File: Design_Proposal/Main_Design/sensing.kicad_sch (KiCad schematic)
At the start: 13 parts, among them IC2 TMP102AIDRLR, J10 Conn_01x03_Male, J11 Conn_01x05_Male

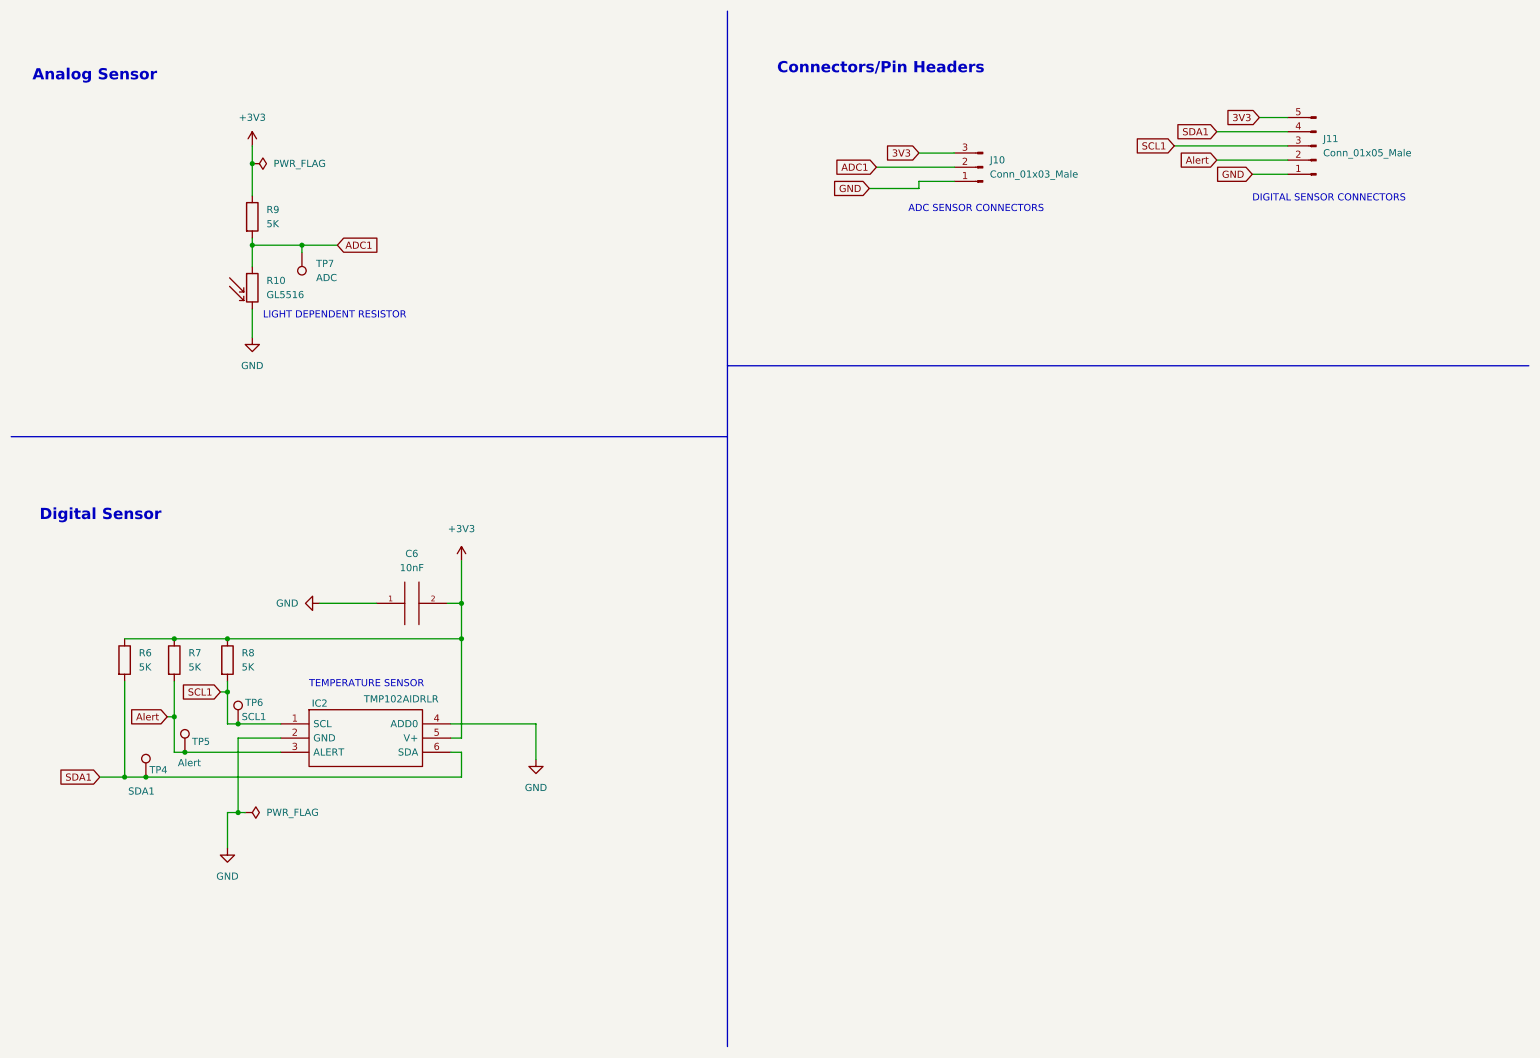
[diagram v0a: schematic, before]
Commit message: Final PCB Design
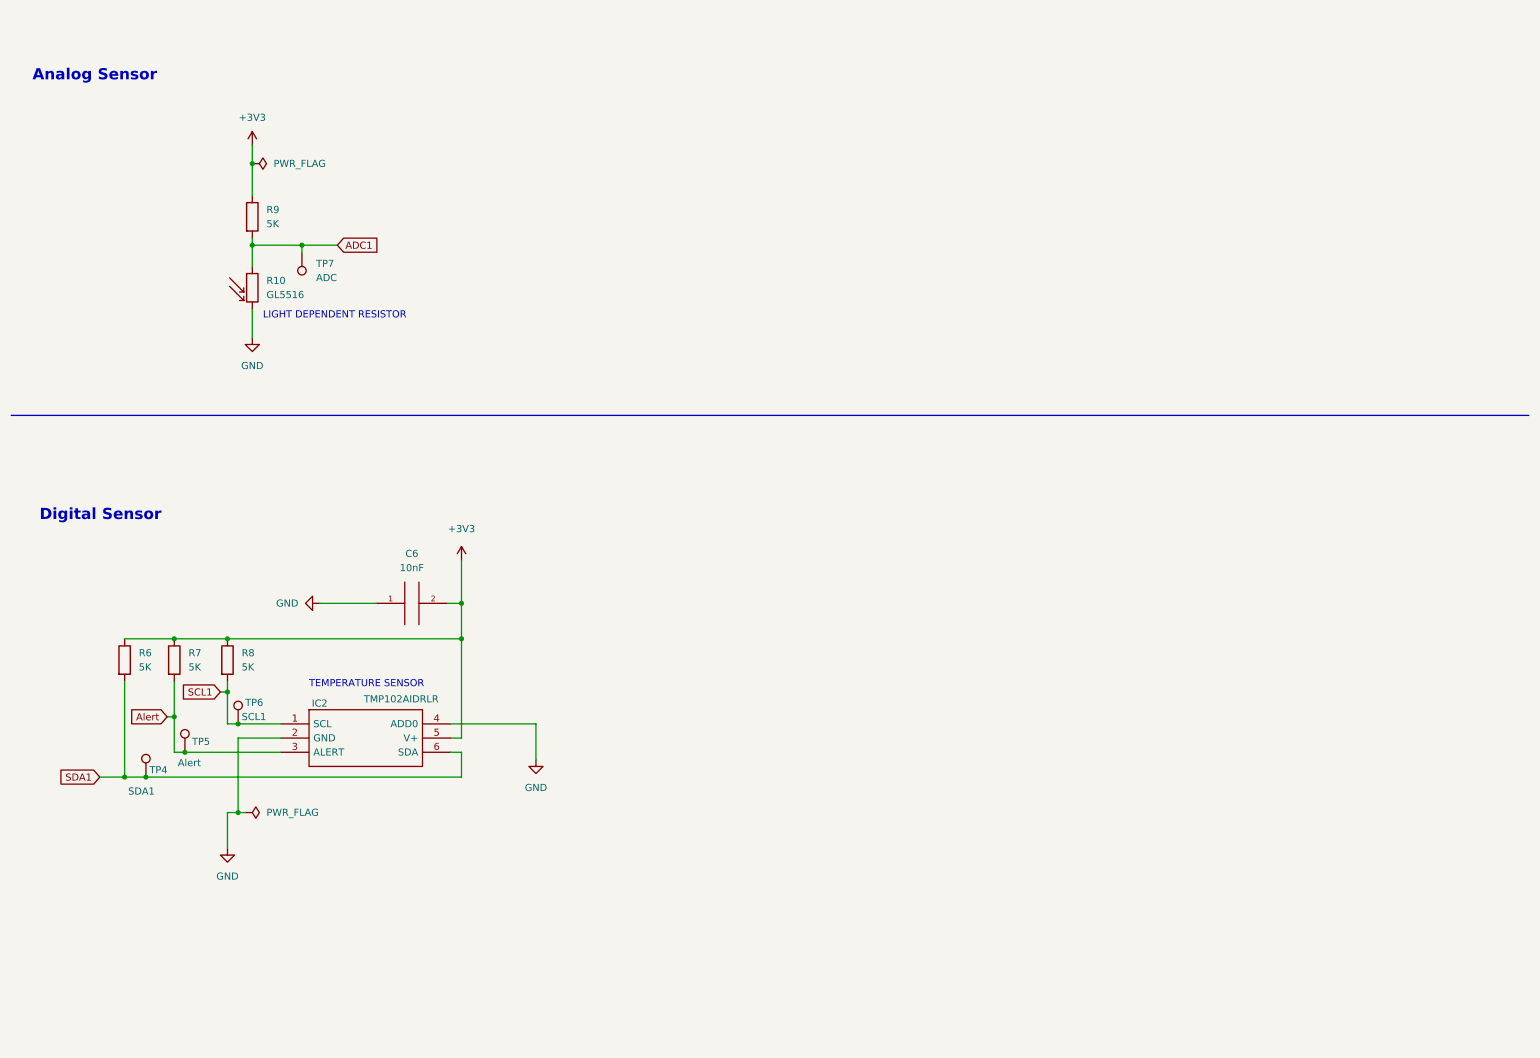
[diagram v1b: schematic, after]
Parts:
- removed J10: Conn_01x03_Male, Connector_PinHeader_2.54mm:PinHeader_1x03_P2.54mm_Vertical, symbol Connector:Conn_01x03_Male
- removed J11: Conn_01x05_Male, Connector_PinHeader_2.54mm:PinHeader_1x05_P2.54mm_Vertical, symbol Connector:Conn_01x05_Male
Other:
- note removed: "ADC SENSOR CONNECTORS"
- note removed: "Connectors/Pin Headers"
- note removed: "DIGITAL SENSOR CONNECTORS"
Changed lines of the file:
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@@
     (stroke (width 0) (type default) (color 0 0 0 0))
   )
-  (wire (pts (xy 236.22 31.75) (xy 241.3 31.75))
-    (stroke (width 0) (type default) (color 0 0 0 0))
-  )
-  (wire (pts (xy 166.37 44.45) (xy 175.26 44.45))
-    (stroke (width 0) (type default) (color 0 0 0 0))
-  )
-  (polyline (pts (xy 140.97 76.2) (xy 284.48 76.2))
+  (polyline (pts (xy 12.7 85.09) (xy 284.48 85.09))
     (stroke (width 0) (type default) (color 0 0 0 0))
   )
@@
     (stroke (width 0) (type default) (color 0 0 0 0))
   )
-  (wire (pts (xy 175.26 43.18) (xy 181.61 43.18))
-    (stroke (width 0) (type default) (color 0 0 0 0))
-  )
   (wire (pts (xy 93.345 118.745) (xy 93.345 125.095))
     (stroke (width 0) (type default) (color 0 0 0 0))
   )
-  (wire (pts (xy 228.6 34.29) (xy 241.3 34.29))
-    (stroke (width 0) (type default) (color 0 0 0 0))
-  )
   (wire (pts (xy 50.165 134.62) (xy 51.435 134.62))
     (stroke (width 0) (type default) (color 0 0 0 0))
@@
     (stroke (width 0) (type default) (color 0 0 0 0))
   )
-  (wire (pts (xy 234.95 41.91) (xy 241.3 41.91))
-    (stroke (width 0) (type default) (color 0 0 0 0))
-  )
   (wire (pts (xy 33.02 149.86) (xy 33.02 132.715))
     (stroke (width 0) (type default) (color 0 0 0 0))
@@
     (stroke (width 0) (type default) (color 0 0 0 0))
   )
-  (wire (pts (xy 167.64 40.64) (xy 181.61 40.64))
-    (stroke (width 0) (type default) (color 0 0 0 0))
-  )
   (wire (pts (xy 55.88 66.04) (xy 55.88 71.12))
     (stroke (width 0) (type default) (color 0 0 0 0))
   )
-  (wire (pts (xy 175.26 38.1) (xy 181.61 38.1))
-    (stroke (width 0) (type default) (color 0 0 0 0))
-  )
   (wire (pts (xy 41.91 139.065) (xy 41.91 145.415))
     (stroke (width 0) (type default) (color 0 0 0 0))
@@
     (stroke (width 0) (type default) (color 0 0 0 0))
   )
-  (wire (pts (xy 228.6 39.37) (xy 241.3 39.37))
-    (stroke (width 0) (type default) (color 0 0 0 0))
-  )
-  (polyline (pts (xy 140.97 88.9) (xy 140.97 198.12))
-    (stroke (width 0) (type default) (color 0 0 0 0))
-  )
   (wire (pts (xy 43.815 145.415) (xy 60.96 145.415))
     (stroke (width 0) (type default) (color 0 0 0 0))
@@
     (stroke (width 0) (type default) (color 0 0 0 0))
   )
-  (polyline (pts (xy 12.7 88.9) (xy 140.97 88.9))
-    (stroke (width 0) (type default) (color 0 0 0 0))
-  )
   (wire (pts (xy 51.435 140.335) (xy 53.34 140.335))
     (stroke (width 0) (type default) (color 0 0 0 0))
   )
-  (polyline (pts (xy 140.97 12.7) (xy 140.97 88.9))
-    (stroke (width 0) (type default) (color 0 0 0 0))
-  )
   (wire (pts (xy 55.88 54.61) (xy 55.88 58.42))
     (stroke (width 0) (type default) (color 0 0 0 0))
   )
-  (wire (pts (xy 175.26 44.45) (xy 175.26 43.18))
-    (stroke (width 0) (type default) (color 0 0 0 0))
-  )
   (wire (pts (xy 93.345 149.86) (xy 93.345 145.415))
-    (stroke (width 0) (type default) (color 0 0 0 0))
-  )
-  (wire (pts (xy 220.98 36.83) (xy 241.3 36.83))
     (stroke (width 0) (type default) (color 0 0 0 0))
   )
@@
     (effects (font (size 1.27 1.27)) (justify left bottom))
   )
-  (text "Connectors/Pin Headers" (at 149.86 24.13 0)
-    (effects (font (size 2 2) bold) (justify left bottom))
-  )
-  (text "ADC SENSOR CONNECTORS\n" (at 173.355 48.895 0)
-    (effects (font (size 1.27 1.27)) (justify left bottom))
-  )
-  (text "DIGITAL SENSOR CONNECTORS\n" (at 234.95 46.99 0)
-    (effects (font (size 1.27 1.27)) (justify left bottom))
-  )
   (text "Analog Sensor\n" (at 16.51 25.4 0)
     (effects (font (size 2 2) bold) (justify left bottom))
-  )
-  (global_label "3V3" (shape input) (at 175.26 38.1 180) (fields_autoplaced)
-    (effects (font (size 1.27 1.27)) (justify right))
-    (property "Intersheet References" "${INTERSHEET_REFS}" (id 0) (at 169.3393 38.1794 0)
-      (effects (font (size 1.27 1.27)) (justify right) hide)
-    )
   )
   (global_label "Alert" (shape input) (at 40.64 139.065 180) (fields_autoplaced)
@@
     )
   )
-  (global_label "ADC1" (shape input) (at 167.64 40.64 180) (fields_autoplaced)
-    (effects (font (size 1.27 1.27)) (justify right))
-    (property "Intersheet References" "${INTERSHEET_REFS}" (id 0) (at 160.3888 40.7194 0)
-      (effects (font (size 1.27 1.27)) (justify right) hide)
-    )
-  )
   (global_label "SDA1" (shape input) (at 28.575 149.86 180) (fields_autoplaced)
     (effects (font (size 1.27 1.27)) (justify right))
@@
     )
   )
-  (global_label "Alert" (shape input) (at 228.6 39.37 180) (fields_autoplaced)
-    (effects (font (size 1.27 1.27)) (justify right))
-    (property "Intersheet References" "${INTERSHEET_REFS}" (id 0) (at 221.8326 39.4494 0)
-      (effects (font (size 1.27 1.27)) (justify right) hide)
-    )
-  )
   (global_label "ADC1" (shape input) (at 71.12 54.61 0) (fields_autoplaced)
     (effects (font (size 1.27 1.27)) (justify left))
     (property "Intersheet References" "${INTERSHEET_REFS}" (id 0) (at 78.3712 54.5306 0)
       (effects (font (size 1.27 1.27)) (justify left) hide)
-    )
-  )
-  (global_label "3V3" (shape input) (at 236.22 31.75 180) (fields_autoplaced)
-    (effects (font (size 1.27 1.27)) (justify right))
-    (property "Intersheet References" "${INTERSHEET_REFS}" (id 0) (at 230.2993 31.8294 0)
-      (effects (font (size 1.27 1.27)) (justify right) hide)
-    )
-  )
-  (global_label "GND" (shape input) (at 234.95 41.91 180) (fields_autoplaced)
-    (effects (font (size 1.27 1.27)) (justify right))
-    (property "Intersheet References" "${INTERSHEET_REFS}" (id 0) (at 228.6664 41.9894 0)
-      (effects (font (size 1.27 1.27)) (justify right) hide)
-    )
-  )
-  (global_label "SDA1" (shape input) (at 228.6 34.29 180) (fields_autoplaced)
-    (effects (font (size 1.27 1.27)) (justify right))
-    (property "Intersheet References" "${INTERSHEET_REFS}" (id 0) (at 221.4093 34.3694 0)
-      (effects (font (size 1.27 1.27)) (justify right) hide)
-    )
-  )
-  (global_label "SCL1" (shape input) (at 220.98 36.83 180) (fields_autoplaced)
-    (effects (font (size 1.27 1.27)) (justify right))
-    (property "Intersheet References" "${INTERSHEET_REFS}" (id 0) (at 213.8498 36.9094 0)
-      (effects (font (size 1.27 1.27)) (justify right) hide)
-    )
-  )
-  (global_label "GND" (shape input) (at 166.37 44.45 180) (fields_autoplaced)
-    (effects (font (size 1.27 1.27)) (justify right))
-    (property "Intersheet References" "${INTERSHEET_REFS}" (id 0) (at 160.0864 44.3706 0)
-      (effects (font (size 1.27 1.27)) (justify right) hide)
     )
   )
@@
     (pin "2")
   )
-  (symbol (lib_id "Connector:Conn_01x05_Male") (at 246.38 36.83 180) (unit 1)
-    (in_bom yes) (on_board yes) (fields_autoplaced)
-    (property "Reference" "J11" (id 0) (at 247.65 35.5599 0)
-      (effects (font (size 1.27 1.27)) (justify right))
-    )
-    (property "Value" "Conn_01x05_Male" (id 1) (at 247.65 38.0999 0)
-      (effects (font (size 1.27 1.27)) (justify right))
-    )
-    (property "Footprint" "Connector_PinHeader_2.54mm:PinHeader_1x05_P2.54mm_Vertical" (id 2) (at 246.38 36.83 0)
-      (effects (font (size 1.27 1.27)) hide)
-    )
-    (property "Datasheet" "~" (id 3) (at 246.38 36.83 0)
-      (effects (font (size 1.27 1.27)) hide)
-    )
-    (pin "1")
-    (pin "2")
-    (pin "3")
-    (pin "4")
-    (pin "5")
-  )
   (symbol (lib_id "power:GND") (at 55.88 71.12 0) (unit 1)
     (in_bom yes) (on_board yes) (fields_autoplaced)
@@
     (pin "1")
   )
-  (symbol (lib_id "Connector:Conn_01x03_Male") (at 186.69 40.64 180) (unit 1)
-    (in_bom yes) (on_board yes) (fields_autoplaced)
-    (property "Reference" "J10" (id 0) (at 187.96 39.3699 0)
-      (effects (font (size 1.27 1.27)) (justify right))
-    )
-    (property "Value" "Conn_01x03_Male" (id 1) (at 187.96 41.9099 0)
-      (effects (font (size 1.27 1.27)) (justify right))
-    )
-    (property "Footprint" "Connector_PinHeader_2.54mm:PinHeader_1x03_P2.54mm_Vertical" (id 2) (at 186.69 40.64 0)
-      (effects (font (size 1.27 1.27)) hide)
-    )
-    (property "Datasheet" "~" (id 3) (at 186.69 40.64 0)
-      (effects (font (size 1.27 1.27)) hide)
-    )
-    (pin "1")
-    (pin "2")
-    (pin "3")
-  )
   (symbol (lib_id "Device:R") (at 55.88 49.53 0) (unit 1)
